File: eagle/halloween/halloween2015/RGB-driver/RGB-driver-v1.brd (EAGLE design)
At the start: 71.7 x 53 mm, 37 parts, among them IC1 MEGA8-AI, J1 RJ12RIGHTANGLE-I2C, J2 RJ12RIGHTANGLE-I2C, Q1 BSP75, Q10 BSP75, Q11 BSP75, Q12 BSP75, Q13 BSP75, Q14 BSP75, Q15 BSP75, Q16 BSP75, Q17 BSP75, Q18 BSP75, Q2 BSP75, Q3 BSP75, Q4 BSP75, Q5 BSP75, Q6 BSP75, Q7 BSP75, Q8 BSP75, Q9 BSP75

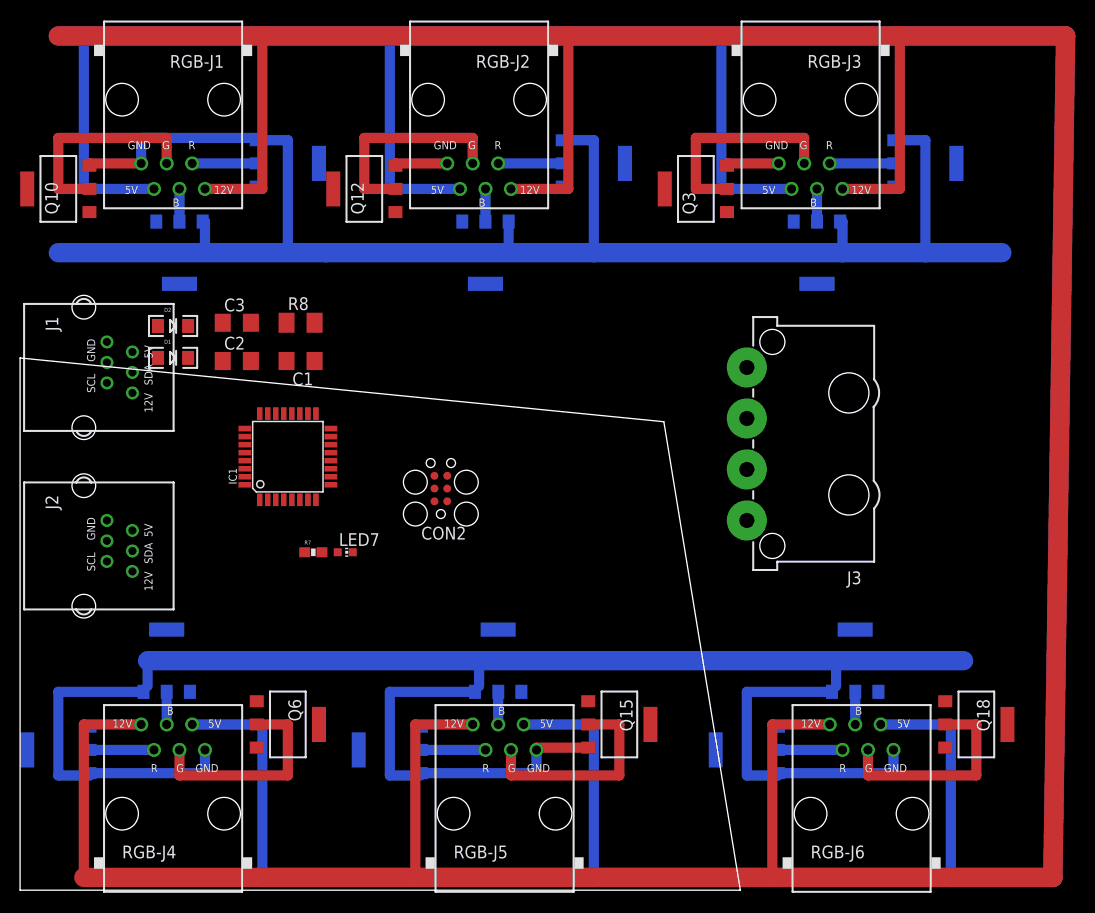
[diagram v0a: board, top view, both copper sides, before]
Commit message: Update
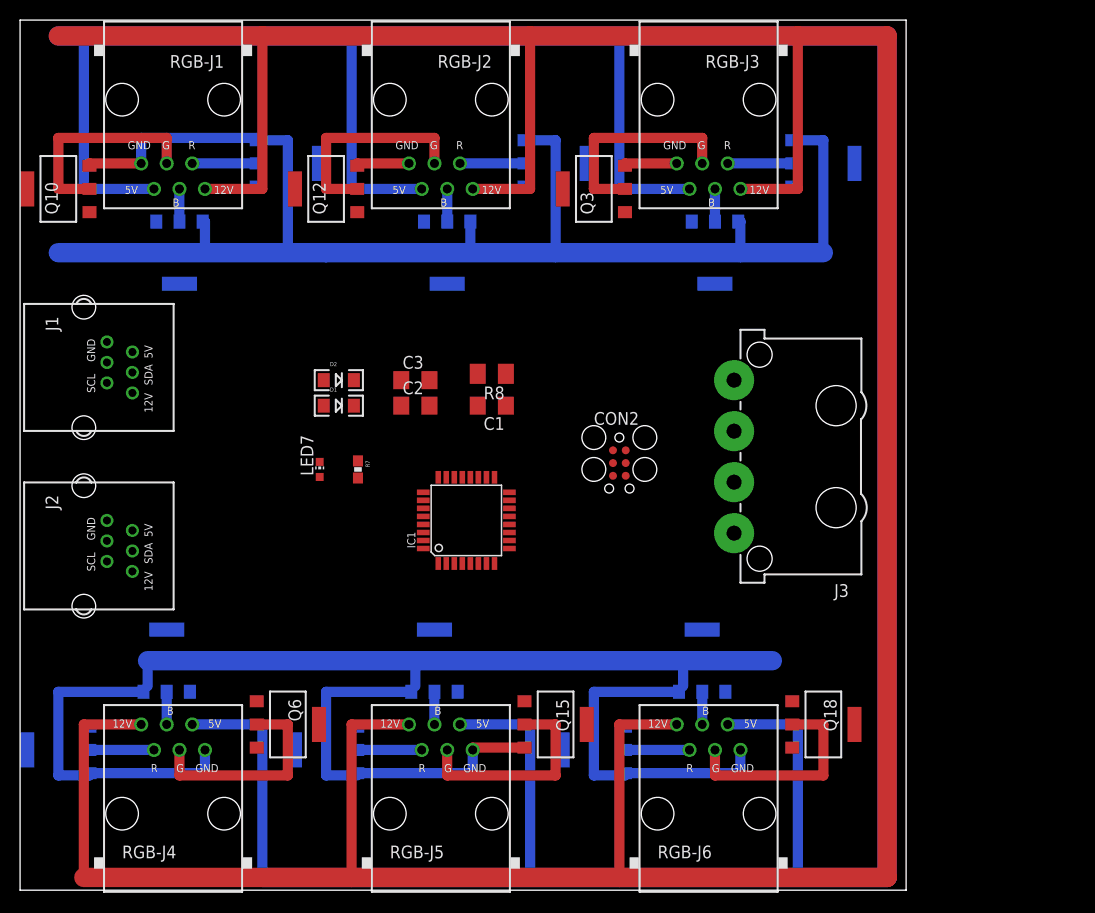
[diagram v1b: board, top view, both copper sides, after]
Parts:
- moved R8 19.7 mm to (47.0, 51.4), turned to 180 degrees
- moved C1 19.6 mm to (47.0, 48.3)
- moved CON2 19.3 mm to (59.7, 45.1), turned to 270 degrees
- moved IC1 18.9 mm to (44.5, 36.8)
- moved C3 18.7 mm to (39.4, 50.8)
- moved C2 18.3 mm to (39.4, 48.3)
- moved D2 17.4 mm to (31.8, 50.8)
- moved D1 17.2 mm to (31.8, 48.3)
- moved Q17 15.2 mm to (67.9, 22.9)
- moved Q16 15.2 mm to (57.1, 14.0)
- moved Q18 15.2 mm to (80.0, 16.5)
- moved RGB-J6 15.2 mm to (68.6, 7.62)
- moved Q3 10.2 mm to (57.1, 69.8)
- moved Q1 10.2 mm to (80.0, 72.4)
- moved Q2 10.2 mm to (69.2, 63.5)
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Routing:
- net N$25: track 396.2 -> 362.0 mm
- net +12V_HP: track 406.4 -> 372.1 mm
- net N$18: track 83.8 -> 64.8 mm
- net N$22: track 288.9 -> 271.2 mm
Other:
- board size 71.7 x 53 mm -> 88.3 x 86.7 mm
